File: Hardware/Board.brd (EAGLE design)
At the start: 100 x 80 mm, 55 parts, among them U1 EDISON_CONNECTOR_FULLMOUNTING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, U2 LAN9512-JZX, U4 EDISON_CONNECTOR_FULLHEADER, X1 J1011F01P

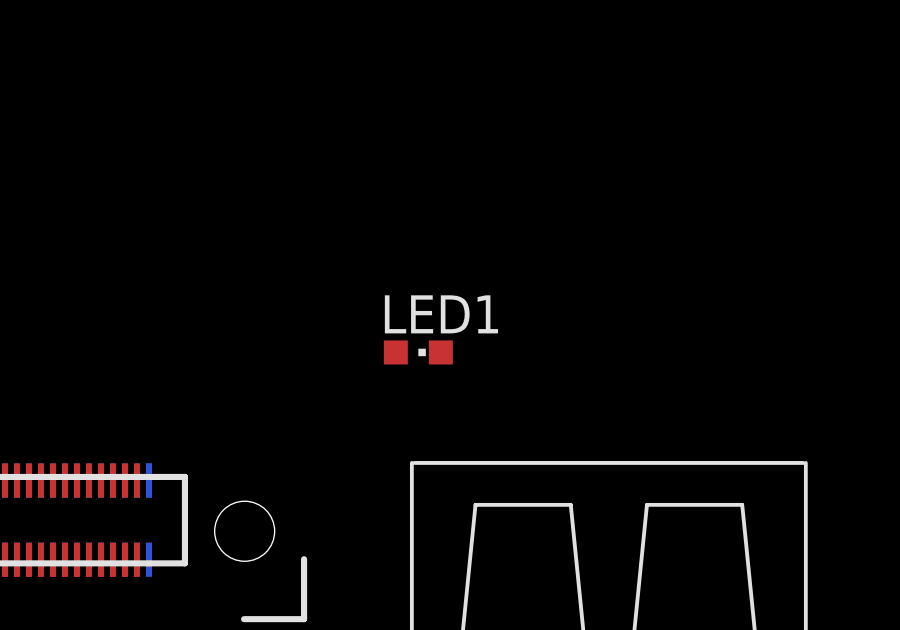
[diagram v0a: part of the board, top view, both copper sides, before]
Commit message: Rolled back previous change
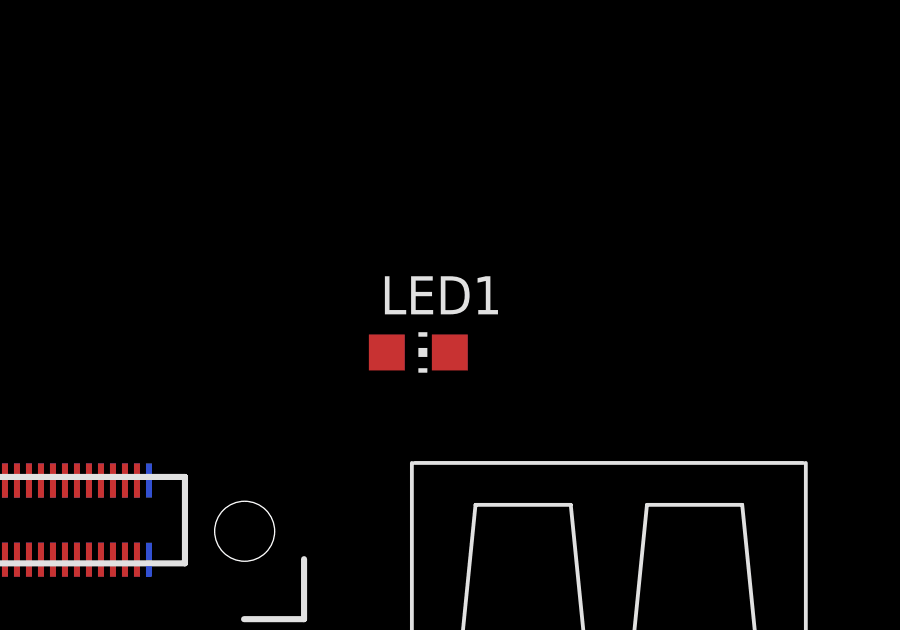
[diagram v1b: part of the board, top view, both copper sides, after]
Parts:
- LED1: device led:CHIPLED_0603 -> led:CHIP-LED0805
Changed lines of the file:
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@@
 <element name="L1" library="murata-inductors" package="L0603" value="2.0A 120Ohm" x="62.23" y="60.96" rot="R270"/>
 <element name="L2" library="murata-inductors" package="L0603" value="2.0A 120Ohm" x="71.12" y="13.97" rot="R270"/>
-<element name="LED1" library="led" package="CHIPLED_0603" value="Green LED" x="41.91" y="62.23" rot="R270"/>
+<element name="LED1" library="led" package="CHIP-LED0805" value="Green LED" x="41.91" y="62.23" rot="R270"/>
 <element name="R1" library="resistor" package="R0603" value="10K" x="76.2" y="41.91" rot="R270"/>
 <element name="R10" library="resistor" package="R1210" value="0" x="63.5" y="33.02" rot="R270"/>
@@
 <contactref element="LED1" pad="C"/>
 <contactref element="U2" pad="20"/>
-<wire x1="45.1358" y1="18.7706" x2="42.66" y2="62.23" width="0" layer="19" extent="1-1"/>
+<wire x1="45.1358" y1="18.7706" x2="42.96" y2="62.23" width="0" layer="19" extent="1-1"/>
 </signal>
 <signal name="N$20">
 <contactref element="LED1" pad="A"/>
 <contactref element="R13" pad="2"/>
-<wire x1="41.16" y1="62.23" x2="76.2" y2="31.1" width="0" layer="19" extent="1-1"/>
+<wire x1="40.86" y1="62.23" x2="76.2" y2="31.1" width="0" layer="19" extent="1-1"/>
 </signal>
 <signal name="N$21">
